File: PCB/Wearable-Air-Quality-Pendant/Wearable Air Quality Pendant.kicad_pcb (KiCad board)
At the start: 2 copper layers, 32.5 x 32.5 mm, 53 parts, among them IC1 MCP73832T-2ACI_MC, IC2 ADPL44002AUJZ, IC3 SGP40-D-R4, J1 USB_C_Receptacle_USB2.0_16P, J2 SWD, J3 UART, Q1 SS8550, U1 STM32U083KCUx

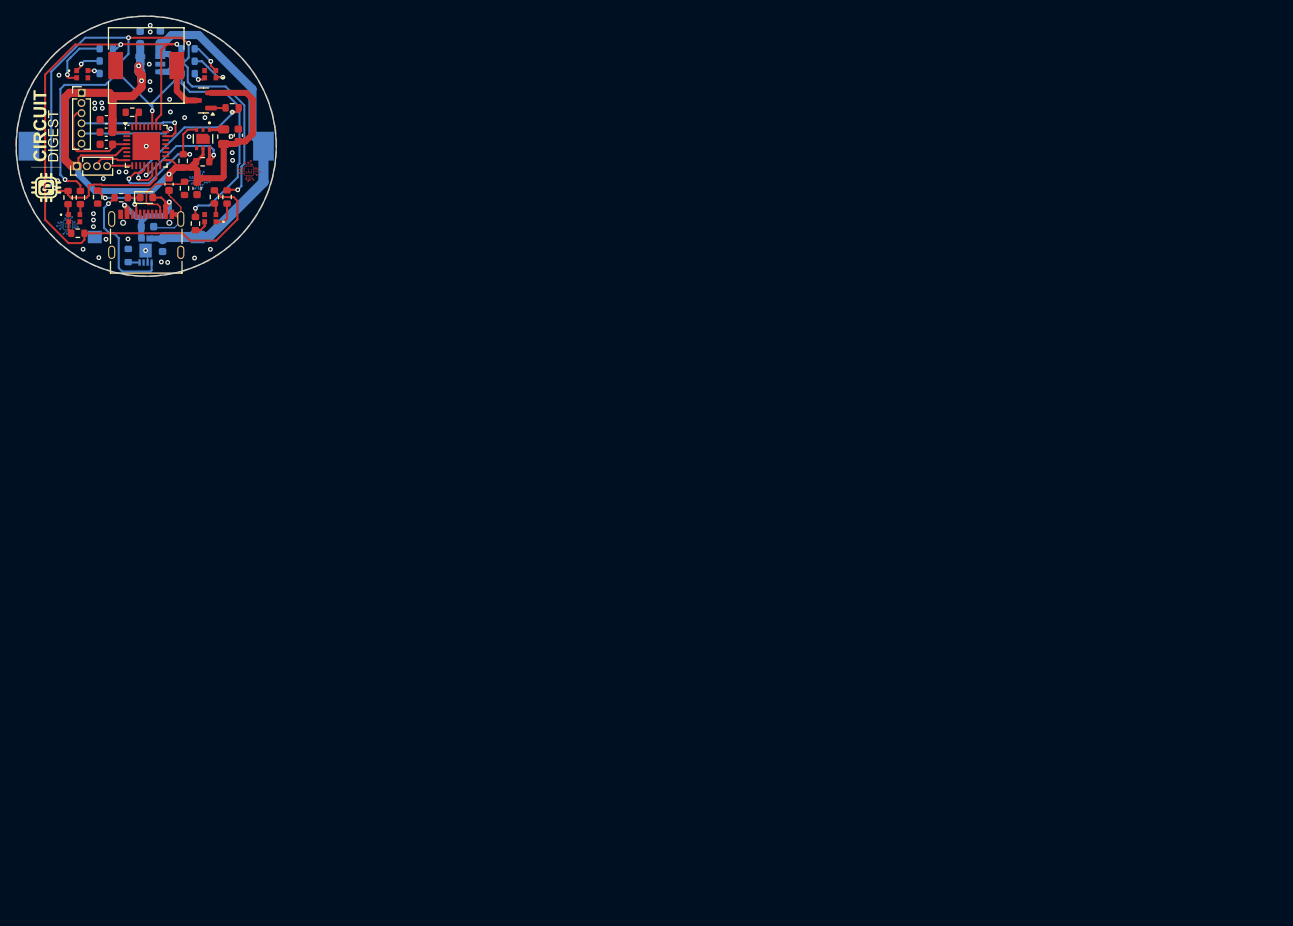
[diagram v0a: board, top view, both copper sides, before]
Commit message: Add files via upload
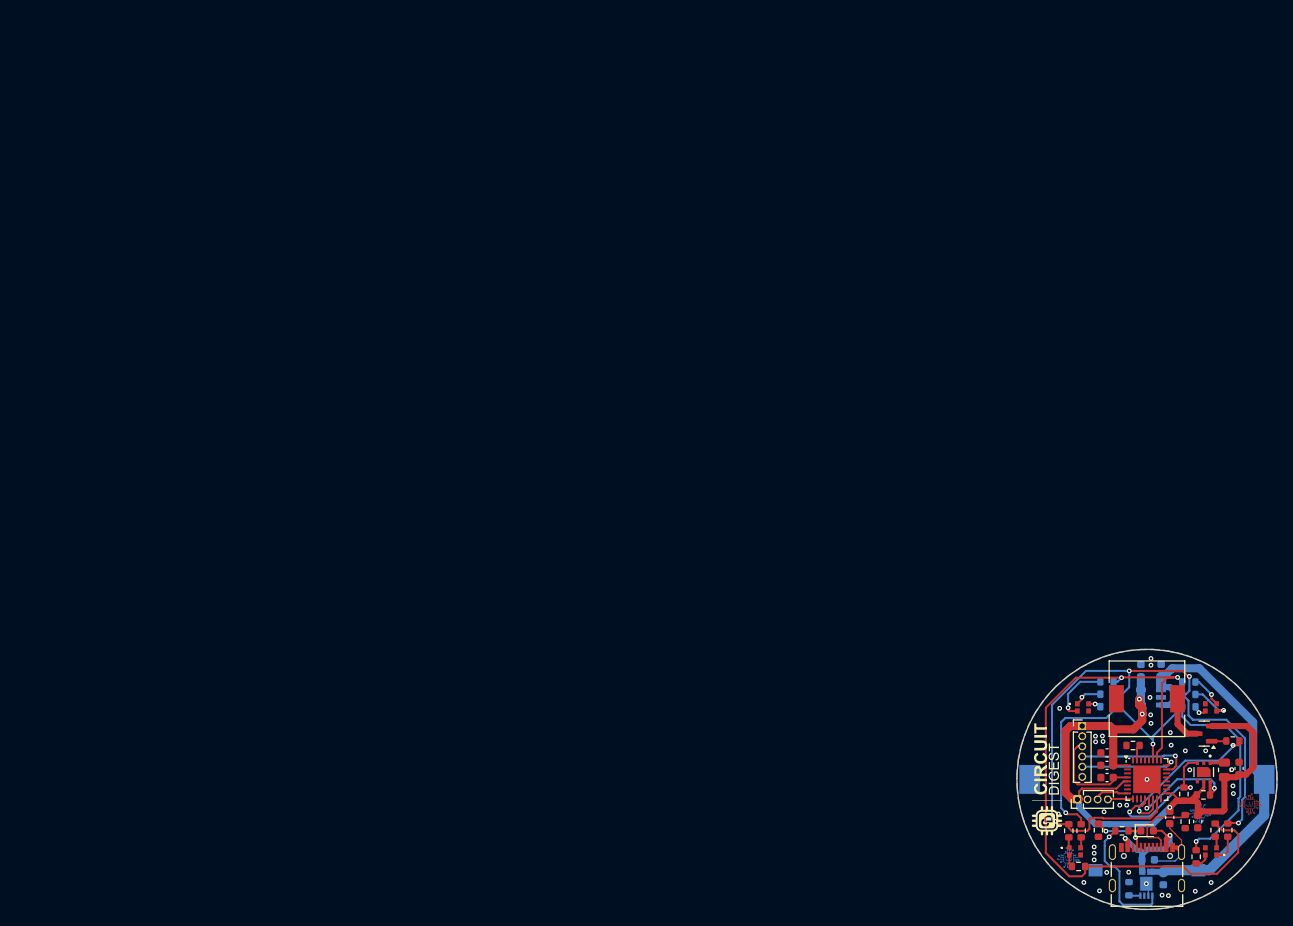
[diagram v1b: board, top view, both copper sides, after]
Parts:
- moved ? 148.0 mm to (131.5, 90.5)
- moved ? 148.0 mm to (117.9, 90.5)
- moved BT1 148.0 mm to (125.1, 79.2)
- moved BZ1 148.0 mm to (125.1, 69.1)
- moved C1 148.0 mm to (125.2, 89.2)
- moved C10 148.0 mm to (120.1, 77.4)
- moved C2 148.0 mm to (127.1, 91.5)
- moved C3 148.0 mm to (126.9, 65.5)
- moved C4 148.0 mm to (124.3, 65.6)
- moved C5 148.0 mm to (136.6, 77.8)
- moved C6 148.0 mm to (127.9, 83.9)
- moved C7 148.0 mm to (131.4, 84.4)
- moved C8 148.0 mm to (120.1, 75.8)
- moved C9 148.0 mm to (120.1, 78.9)
- moved D1 148.0 mm to (125.1, 85.6)
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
